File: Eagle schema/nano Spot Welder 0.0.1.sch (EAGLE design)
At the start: 32 parts, among them Q2 BC548, T1 BTA 41 / 600V, U1 NANO, U2 DISPLAY-NOKIA-5110, U3 DS18B20, X3 ~230V, X4 Mikro trafó

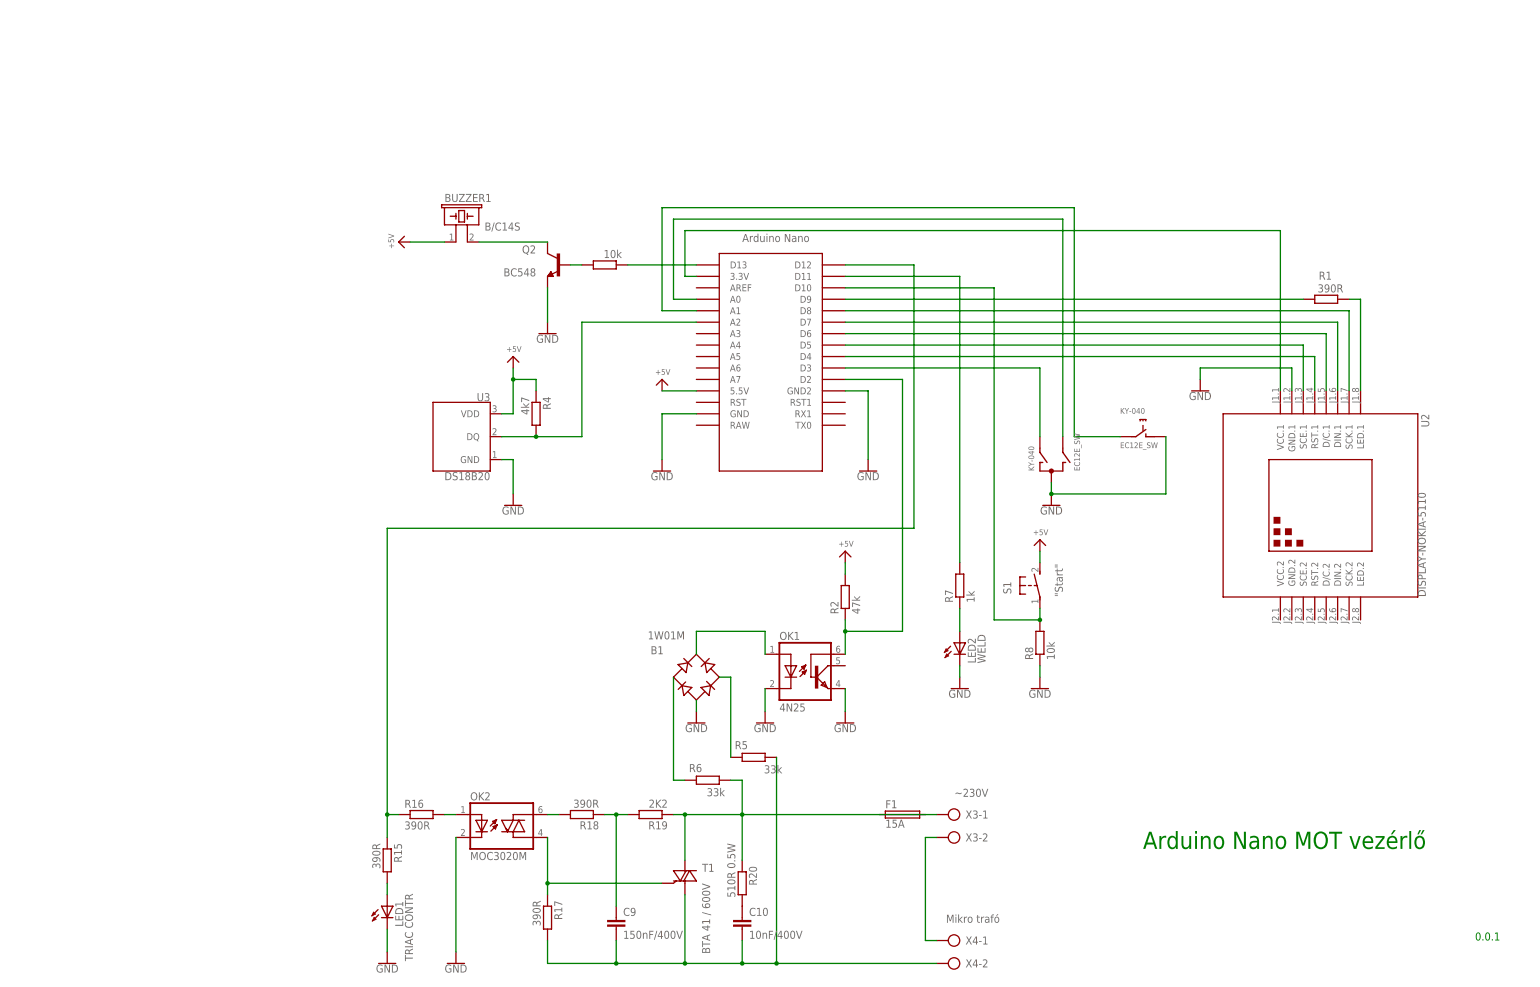
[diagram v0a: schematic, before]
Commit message: - átszervezés
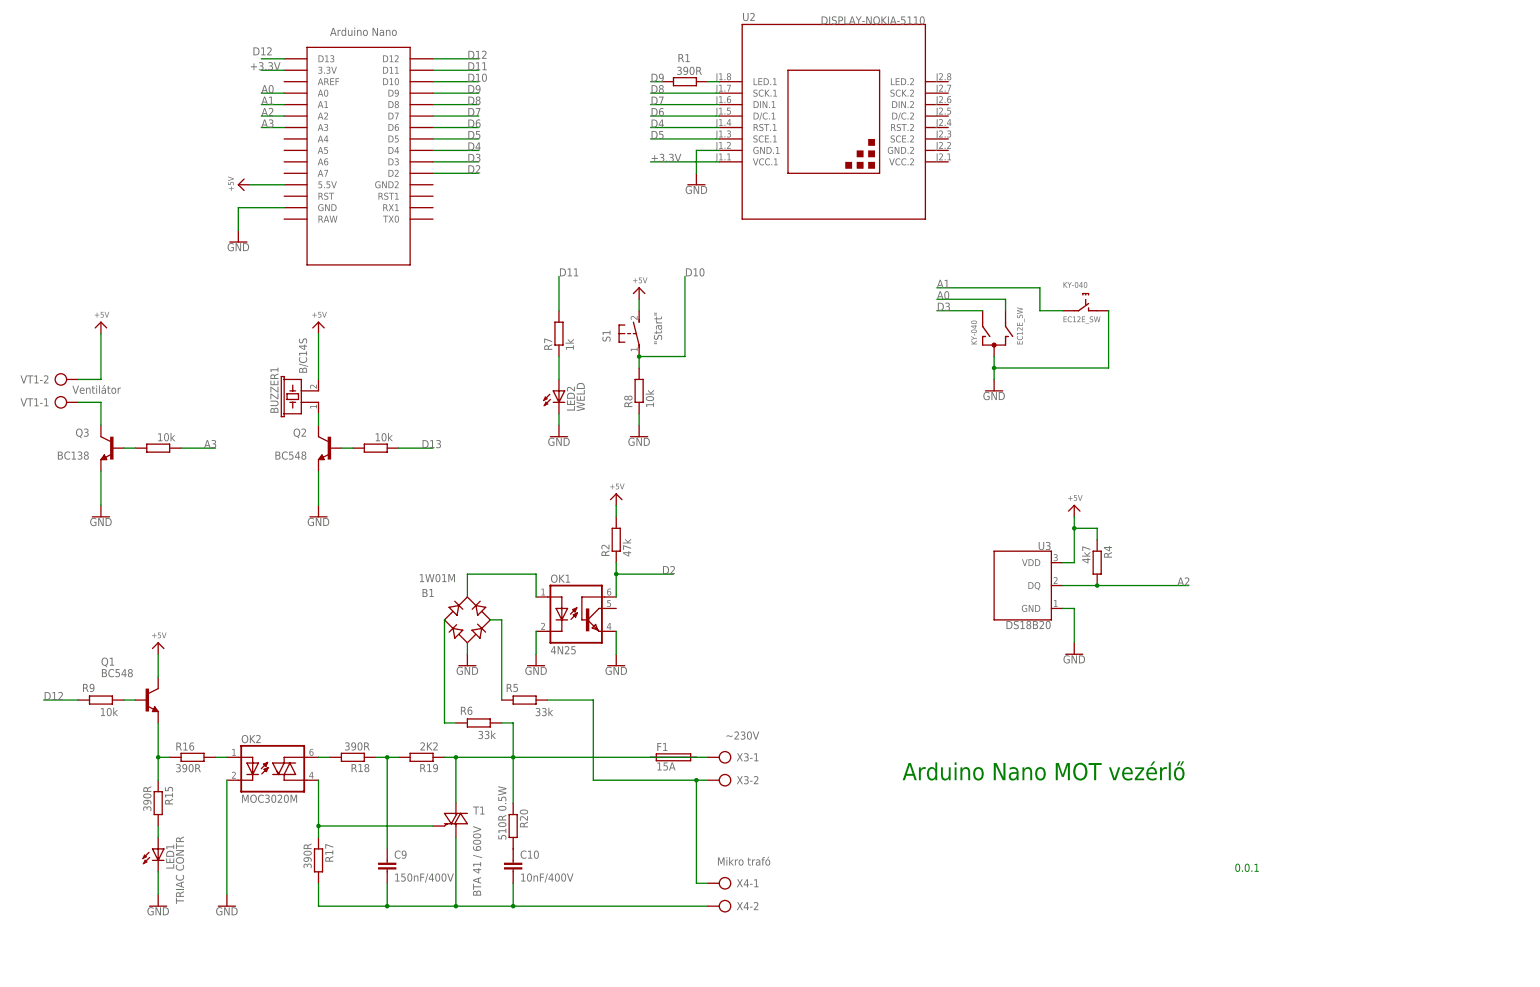
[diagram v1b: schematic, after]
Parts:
- added Q1: BC548, transistor-npn:BC548
- added Q3: BC138, transistor-npn:BC548
- added R10, R9: 10k, resistor:R-EU_0204/7
- added VT1: Ventilátor, con-ptr500:AK300/2
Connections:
- net N$10 renamed A2
- net N$12 renamed A0
- net N$13 renamed D10
- net N$14 renamed +3.3V
- net N$2 renamed D9
- net N$27 renamed A1
- net N$3 renamed D8
- net N$30 renamed D11
- net N$4 renamed D7
- net N$5 renamed D6
- net N$6 renamed D5
- net N$7 renamed D4
- net N$8 renamed D3
- net N$9 renamed D2
- removed net N$11: R3.1, U1.D13
- removed net N$17: BUZZER1.2, Q2.C
- new net A3: R10.1, U1.A3
- new net D12: R9.2, U1.D12, U1.D13
- new net D13: R3.1
- new net N$3: BUZZER1.1, Q2.C
- new net N$4: Q1.B, R9.1
- new net N$5: Q3.B, R10.2
- new net N$6: Q3.C, VT1-1.KL
- net GND: now also Q3.E; no longer U1.GND2
- net MOC: now also Q1.E; no longer U1.D12
- net N$28: now also R5.1
- net N$33: no longer R5.1
- net VCC: now also BUZZER1.2, Q1.C, VT1-2.KL; no longer BUZZER1.1
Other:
- moved on the sheet: B1, BUZZER1, C10, C9, F1, KY-040, LED1, LED2, OK1, OK2, Q2, R1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
